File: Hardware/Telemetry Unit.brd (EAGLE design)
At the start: 50.8 x 63.5 mm, 55 parts, among them IC1 MEGA128-A, IC2 FT232RL, J2 503182-1852, J3 10118193-0001LF, Q1 10MHz, U1 MPL3115A2, U2 AP65111A, U3 LSM6DS3

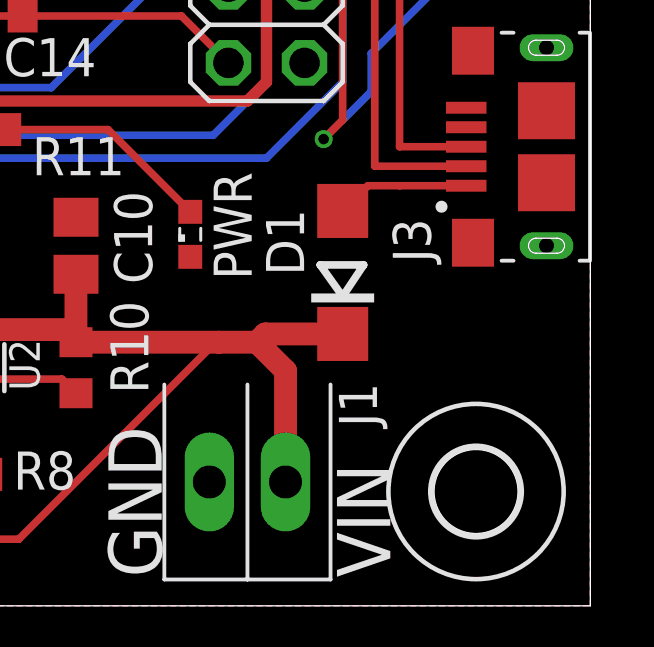
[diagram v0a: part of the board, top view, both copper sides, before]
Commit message: Added fuse to usb
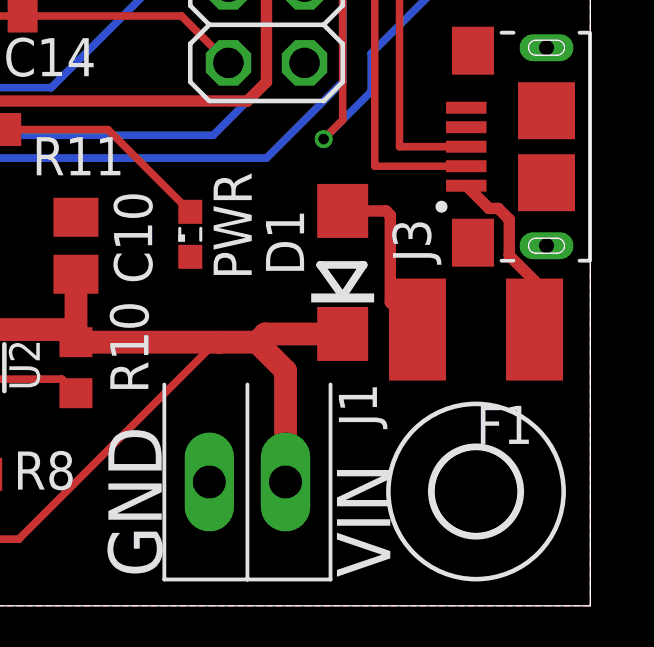
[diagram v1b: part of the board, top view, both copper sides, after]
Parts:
- added F1: MF-MSMF050-2, MF-MSMF050-2:FUSM1812X02
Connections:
- new net N$22: F1.1, J3.1
- net V_USB: now also F1.2; no longer J3.1
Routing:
- net N$22: track 0.00 -> 5.92 mm
- net V_USB: track 4.47 -> 5.83 mm
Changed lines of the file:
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@@
 <?xml version="1.0" encoding="utf-8"?>
 <!DOCTYPE eagle SYSTEM "eagle.dtd">
-<eagle version="9.2.2">
+<eagle version="9.3.0">
 <drawing>
 <settings>
@@
 <attribute name="VALUE" x="30.7975" y="39.6875" size="1.27" layer="27" rot="R180"/>
 </element>
+<element name="F1" library="MF-MSMF050-2" package="FUSM1812X02" value="MF-MSMF050-2" x="46.99" y="9.2075" smashed="yes" rot="R180">
+<attribute name="AVAILABILITY" value="Unavailable" x="46.99" y="9.2075" size="1.778" layer="27" rot="R180" display="off"/>
+<attribute name="DESCRIPTION" value=" PTC Resettable Fuse 0.5A_hold_ 1A_trip_ 15V 100A 0.8W 0.15s 0.15Ohm SMD Solder Pad 1812 T/R " x="46.99" y="9.2075" size="1.778" layer="27" rot="R180" display="off"/>
+<attribute name="MF" value="Bourns" x="46.99" y="9.2075" size="1.778" layer="27" rot="R180" display="off"/>
+<attribute name="MP" value="MF-MSMF050-2" x="46.99" y="9.2075" size="1.778" layer="27" rot="R180" display="off"/>
+<attribute name="NAME" x="48.89605" y="6.666109375" size="1.2707" layer="25" rot="R180"/>
+<attribute name="PACKAGE" value="1812 Bourns" x="46.99" y="9.2075" size="1.778" layer="27" rot="R180" display="off"/>
+<attribute name="PRICE" value="None" x="46.99" y="9.2075" size="1.778" layer="27" rot="R180" display="off"/>
+<attribute name="VALUE" x="48.89841875" y="13.02435" size="1.27228125" layer="27" rot="R180"/>
+</element>
 </elements>
 <signals>
@@
 </signal>
 <signal name="V_USB">
-<contactref element="J3" pad="1"/>
 <contactref element="D1" pad="A"/>
-<wire x1="43.386" y1="14.0035" x2="42.545" y2="13.1625" width="0.254" layer="1"/>
-<wire x1="46.6645" y1="14.0035" x2="44.45" y2="14.0035" width="0.254" layer="1"/>
-<wire x1="44.45" y1="14.0035" x2="43.386" y2="14.0035" width="0.254" layer="1"/>
+<contactref element="F1" pad="2"/>
+<wire x1="45.04" y1="9.2075" x2="44.1325" y2="10.115" width="0.381" layer="1"/>
+<wire x1="44.1325" y1="10.115" x2="44.1325" y2="13.0175" width="0.381" layer="1"/>
+<wire x1="44.1325" y1="13.0175" x2="43.9875" y2="13.1625" width="0.381" layer="1"/>
+<wire x1="43.9875" y1="13.1625" x2="42.545" y2="13.1625" width="0.381" layer="1"/>
 </signal>
 <signal name="N$11">
@@
 <wire x1="38.4175" y1="37.7825" x2="39.09" y2="37.11" width="0.254" layer="1"/>
 </signal>
+<signal name="N$22">
+<contactref element="J3" pad="1"/>
+<contactref element="F1" pad="1"/>
+<wire x1="46.6645" y1="14.0035" x2="47.4216" y2="13.2464" width="0.381" layer="1"/>
+<wire x1="47.4216" y1="13.2464" x2="47.73153125" y2="13.2464" width="0.381" layer="1"/>
+<wire x1="48.94" y1="10.83166875" x2="48.94" y2="9.2075" width="0.381" layer="1"/>
+<wire x1="48.0966" y1="11.67506875" x2="48.94" y2="10.83166875" width="0.381" layer="1"/>
+<wire x1="47.73153125" y1="13.2464" x2="48.0966" y2="12.88133125" width="0.381" layer="1"/>
+<wire x1="48.0966" y1="12.88133125" x2="48.0966" y2="11.67506875" width="0.381" layer="1"/>
+</signal>
 </signals>
 <mfgpreviewcolors>
@@
 <mfgpreviewcolor name="substratecolor" color="0xFF786E46"/>
 </mfgpreviewcolors>
-<errors>
-</errors>
 </board>
 </drawing>
